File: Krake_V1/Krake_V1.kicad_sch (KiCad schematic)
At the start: 63 parts, among them J1 Barrel_Jack_Switch_SMT, Q301 BSS138, U1 LM7805_TO220, U301 PCF8574AT_3_518, U302 LCD_20x4_Character-GPAD_SCH_L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

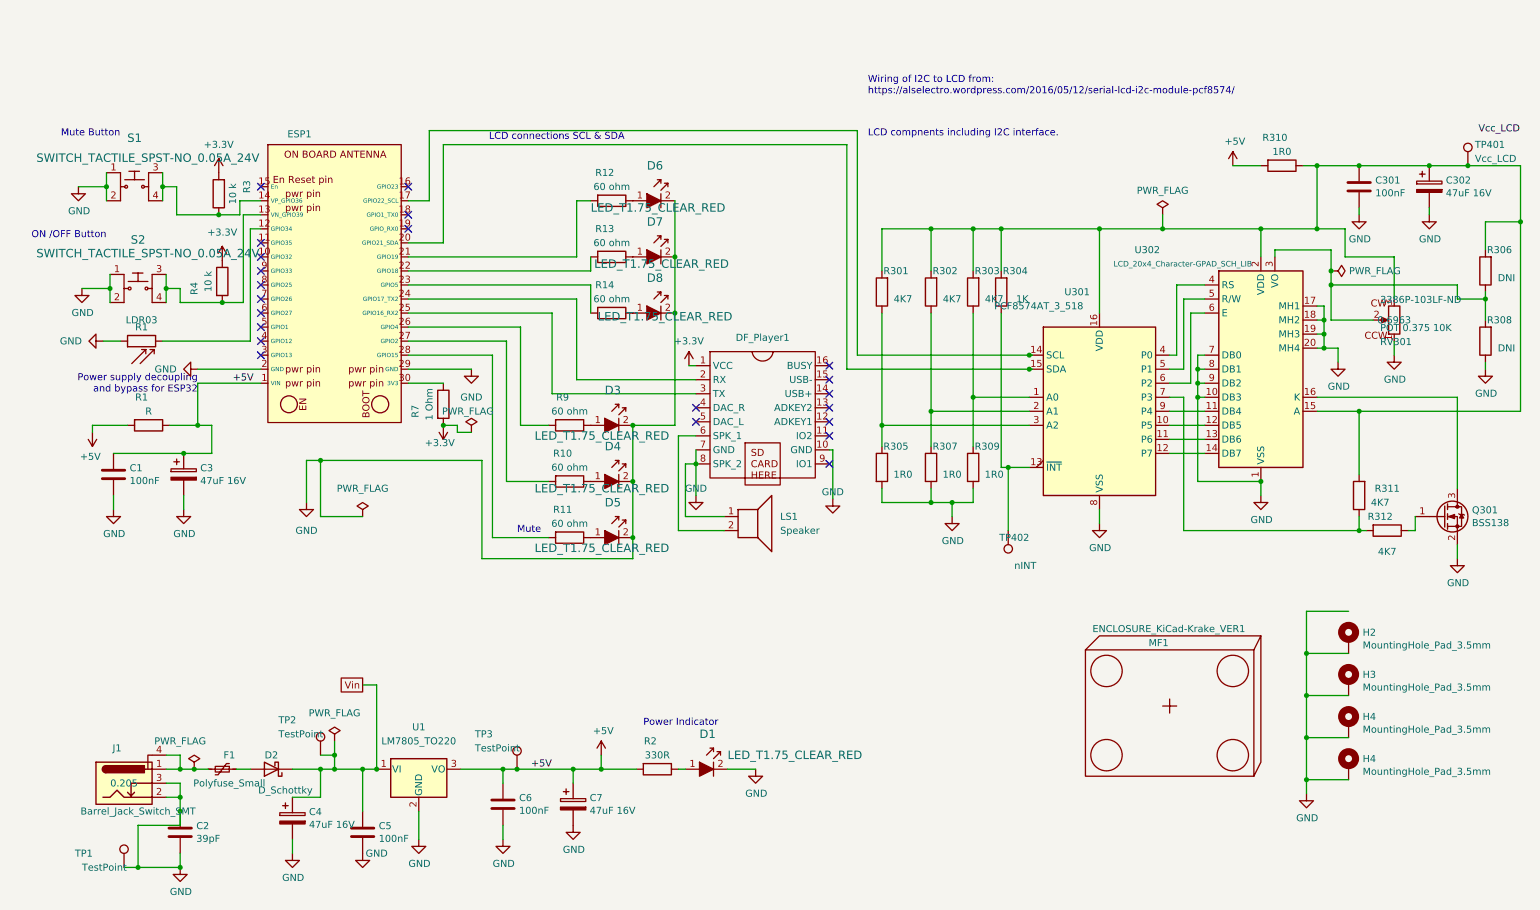
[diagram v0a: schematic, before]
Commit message: Adding Rotary Encoder to Krake
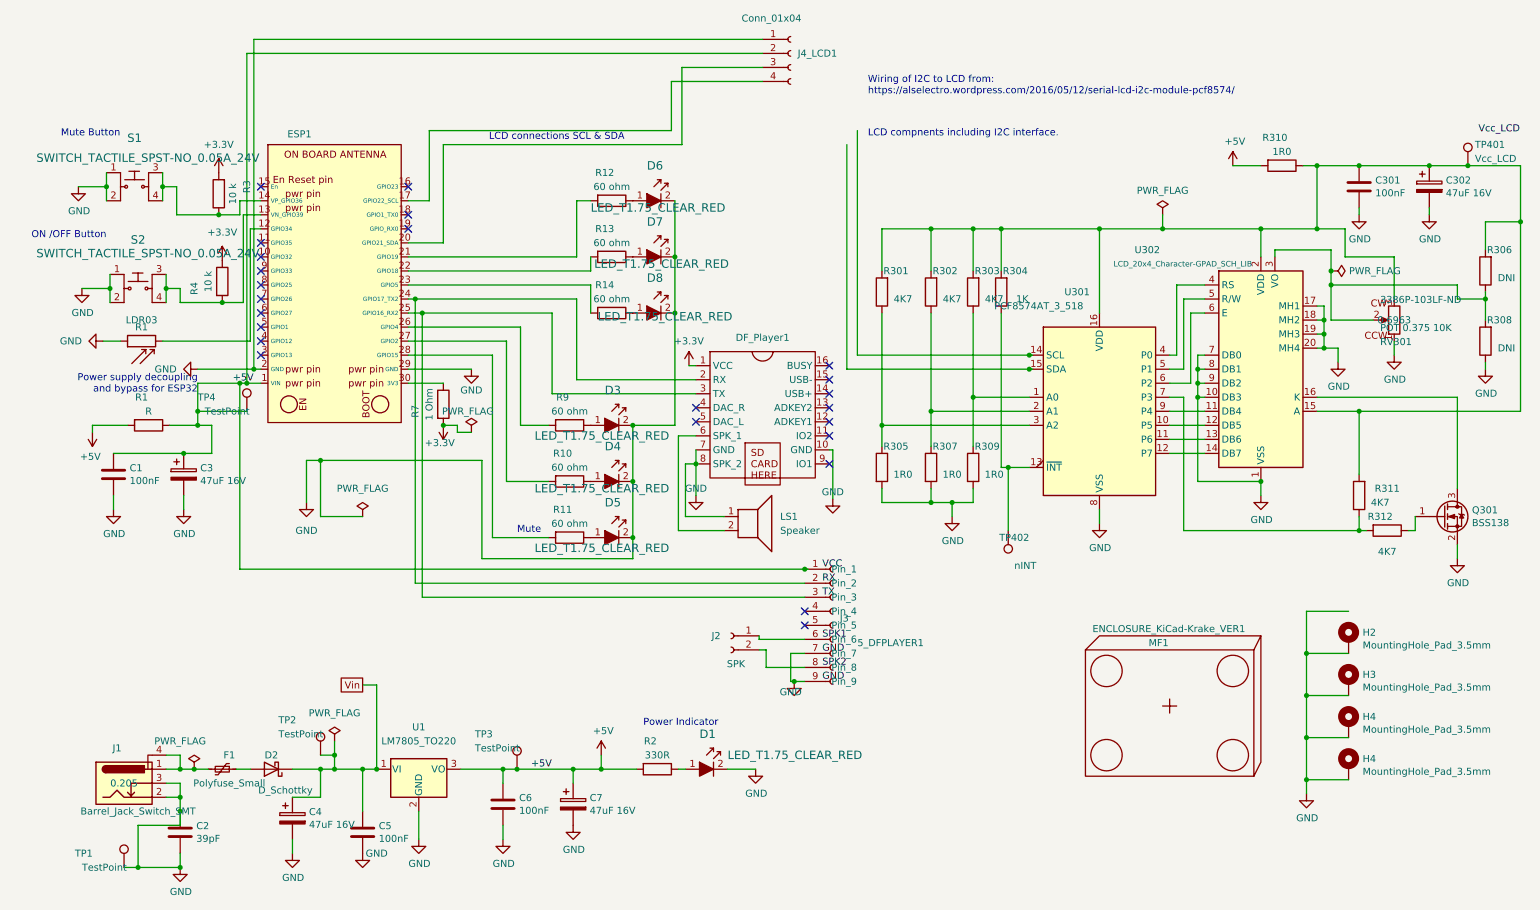
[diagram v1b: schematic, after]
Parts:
- added J2: SPK, Connector_PinHeader_1.27mm:PinHeader_1x02_P1.27mm_Vertical, symbol Connector:Conn_01x02_Socket
- added J3: 5_DFPLAYER1, Connector_PinHeader_1.00mm:PinHeader_1x09_P1.00mm_Vertical, symbol Connector:Conn_01x09_Socket
- added J4_LCD1: Conn_01x04, Connector_PinSocket_2.54mm:PinSocket_1x04_P2.54mm_Vertical, symbol Connector:Conn_01x04_Socket
- added TP4: TestPoint, TestPoint:TestPoint_Loop_D2.54mm_Drill1.5mm_Beaded, symbol Connector:TestPoint
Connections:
- net +5V: now also J3.1 (Pin_1), J4_LCD1.2 (Pin_2), TP4.1
- net GND: now also J3.7 (Pin_7), J3.9 (Pin_9), J4_LCD1.1 (Pin_1)
- net at ESP1.17 (GPIO22_SCL): now also J4_LCD1.4 (Pin_4); no longer U301.14 (SCL)
- net at ESP1.20 (GPIO21_SDA): now also J4_LCD1.3 (Pin_3); no longer U301.15 (SDA)
- net at DF_Player1.2 (RX), ESP1.24 (GPIO17_TX2): now also J3.2 (Pin_2)
- net at DF_Player1.3 (TX), ESP1.25 (GPIO16_RX2): now also J3.3 (Pin_3)
- new net: J2.1 (Pin_1), J3.6 (Pin_6)
- new net: J2.2 (Pin_2), J3.8 (Pin_8)
- no-connect marks 22 -> 24
